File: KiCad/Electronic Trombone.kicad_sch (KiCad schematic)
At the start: 3 parts, among them J1 691137710003

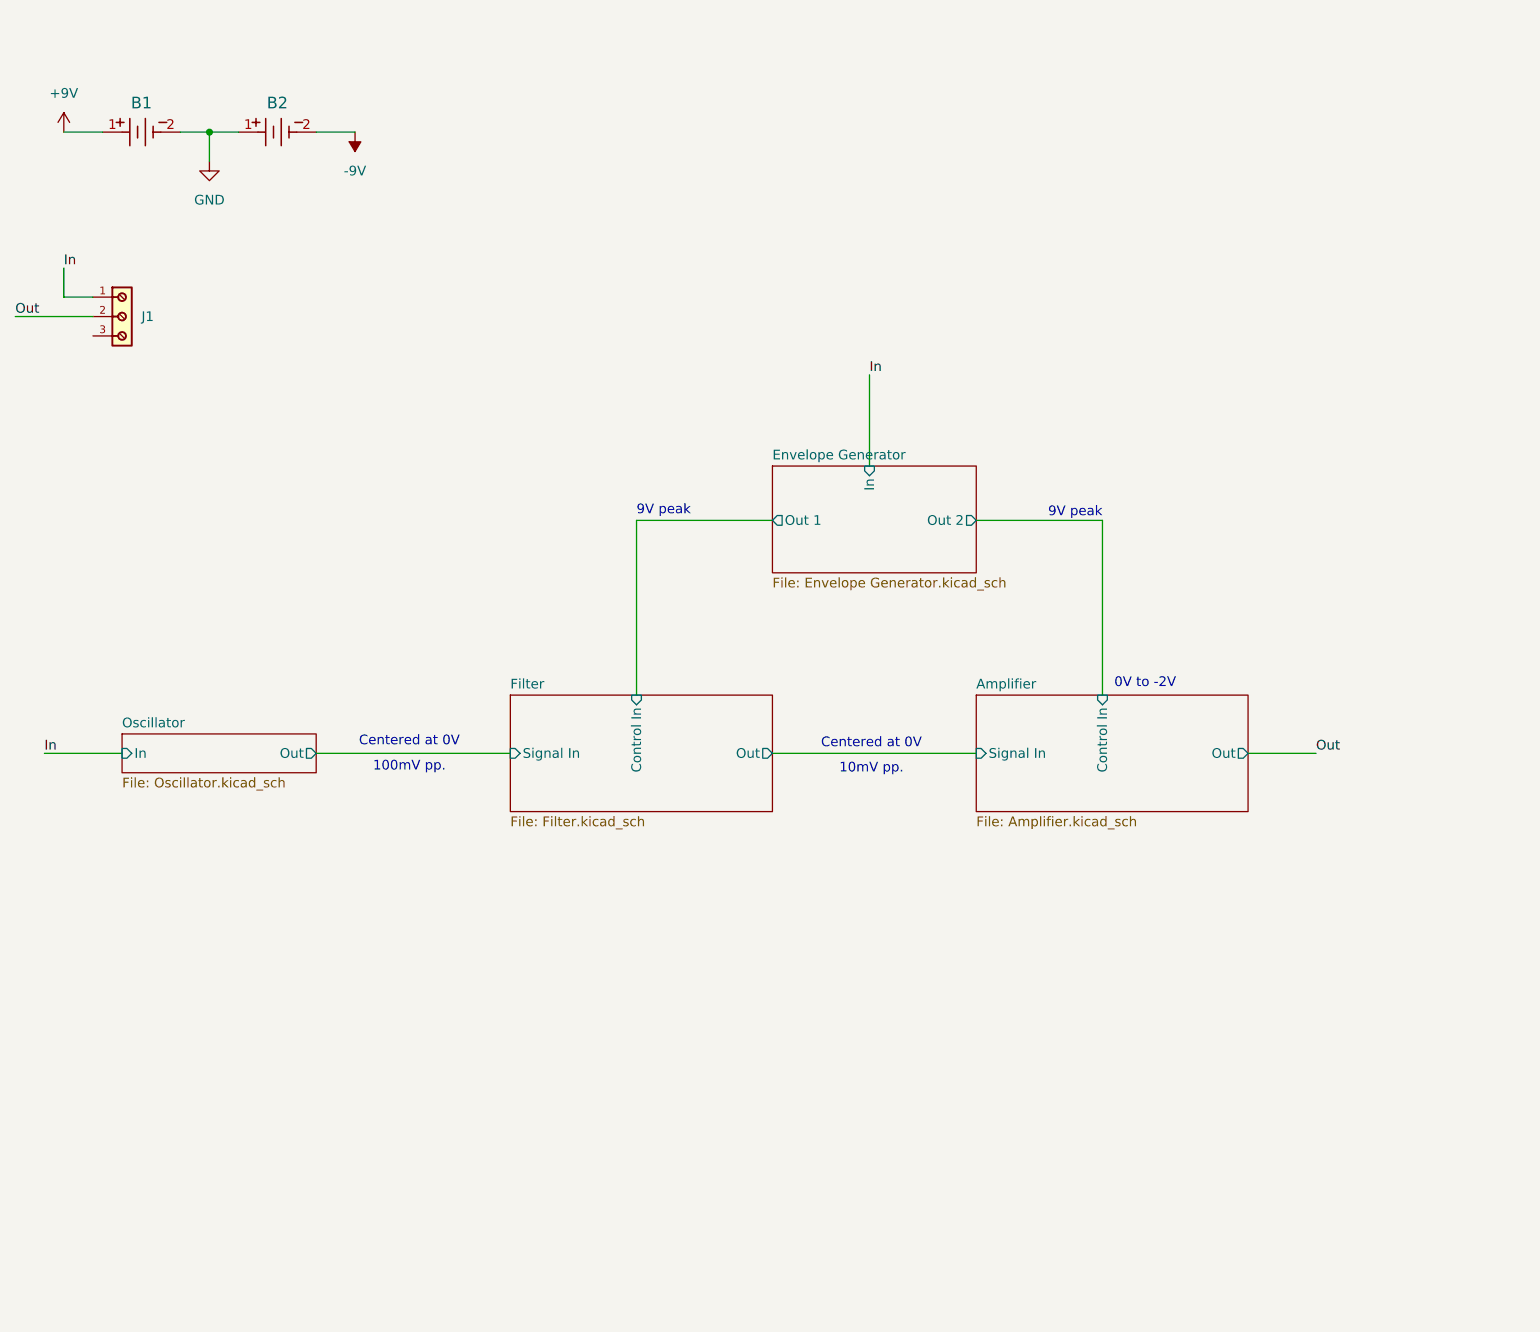
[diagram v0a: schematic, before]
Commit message: finalizing schematic
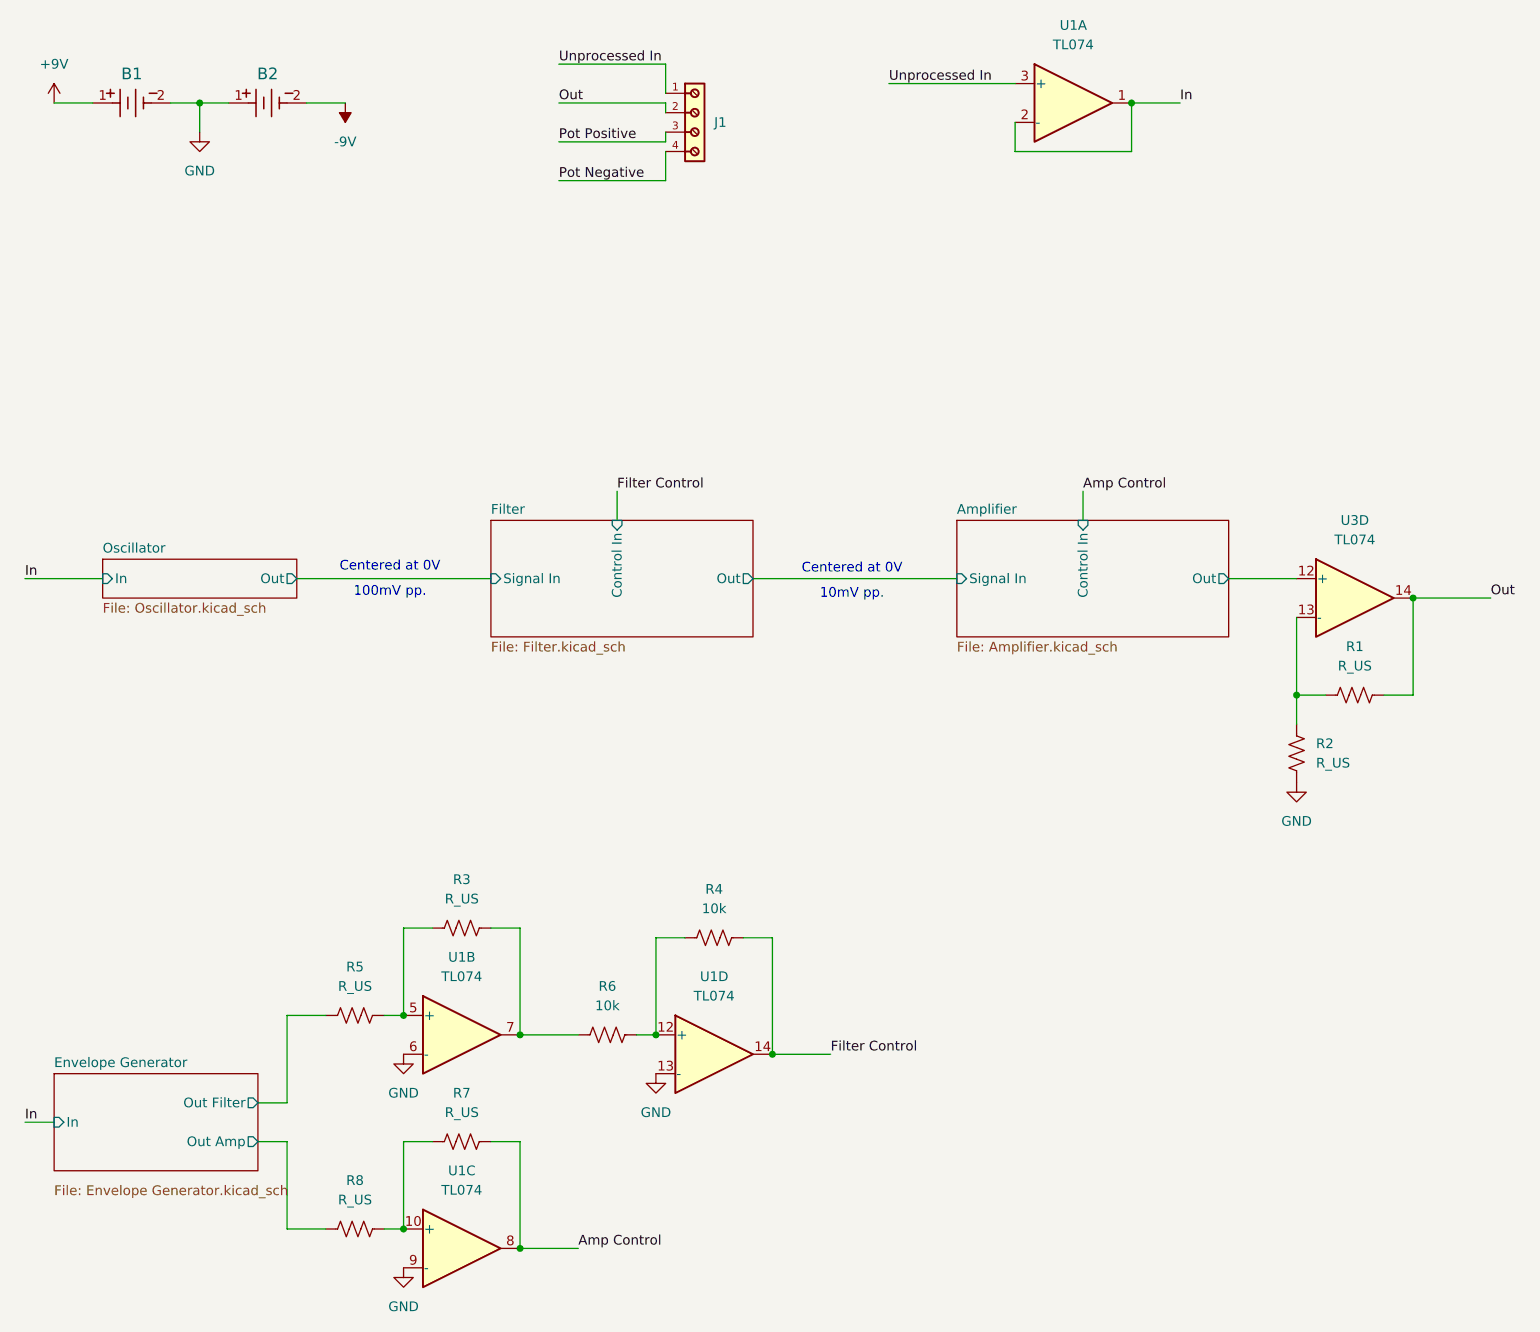
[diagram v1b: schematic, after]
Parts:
- removed J1: 691137710003, 691137710003:691137710003, symbol Header 691137710003:691137710003
- added J1: 691137710004, 691137710004:691137710004, symbol Header 691137710004:691137710004
- added R1, R2, R3, R5, R7, R8: R_US, symbol Device:R_US
- added R4, R6: 10k, symbol Device:R_US
- added U1, U3: TL074, symbol Amplifier_Operational:TL074
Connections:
- net GND: now also R2.1, U1.13 (-), U1.6 (-), U1.9 (-)
- net In: now also U1.1, U1.2 (-)
- net Out: now also J1.2, R1.2, U3.14
- new net: R4.1, R6.2, U1.12 (+)
- new net: R3.1, R5.2, U1.5 (+)
- new net: R3.2, R6.1, U1.7
- new net: R7.1, R8.2, U1.10 (+)
- new net: R1.1, R2.2, U3.13 (-)
- new net Amp Control: R7.2, U1.8
- new net Amplifier/Out: U3.12 (+)
- new net Envelope Generator/Out Amp: R8.1
- new net Envelope Generator/Out Filter: R5.1
- new net Filter Control: R4.2, U1.14
- new net Pot Negative: J1.4
- new net Pot Positive: J1.3
- new net Unprocessed In: J1.1, U1.3 (+)
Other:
- sheet Envelope Generator ports: added Out Amp, Out Filter; removed Out 1, Out 2
- note removed: "0V to -2V"
- note removed: "9V peak"
- moved on the sheet: B1, B2
